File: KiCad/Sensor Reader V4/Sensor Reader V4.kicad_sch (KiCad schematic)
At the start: 33 parts, among them J1 ADS1115_HE_Reader, J10 Conn_01x02_Socket, J11 Conn_01x02_Socket, J12 Conn_01x02_Socket, J13 Conn_01x02_Socket, J14 Conn_01x02_Socket, J15 5V_Input, J16 3.3V_Output, J2 ADS1115_Battery_Voltage, J3 I2C Shifter High, J4 I2C Shifter Low, J5 USB_C_Receptacle_USB2.0_16P, J6 Exposed_UART, J7 Conn_01x02_Socket, J8 Conn_01x02_Socket, J9 Conn_01x02_Socket, SW1 SW_MEC_5E, SW2 SW_MEC_5E, U1 AMS1117-3.3, U2 USBLC6-2P6, U4 ESP32-C3-WROOM-02

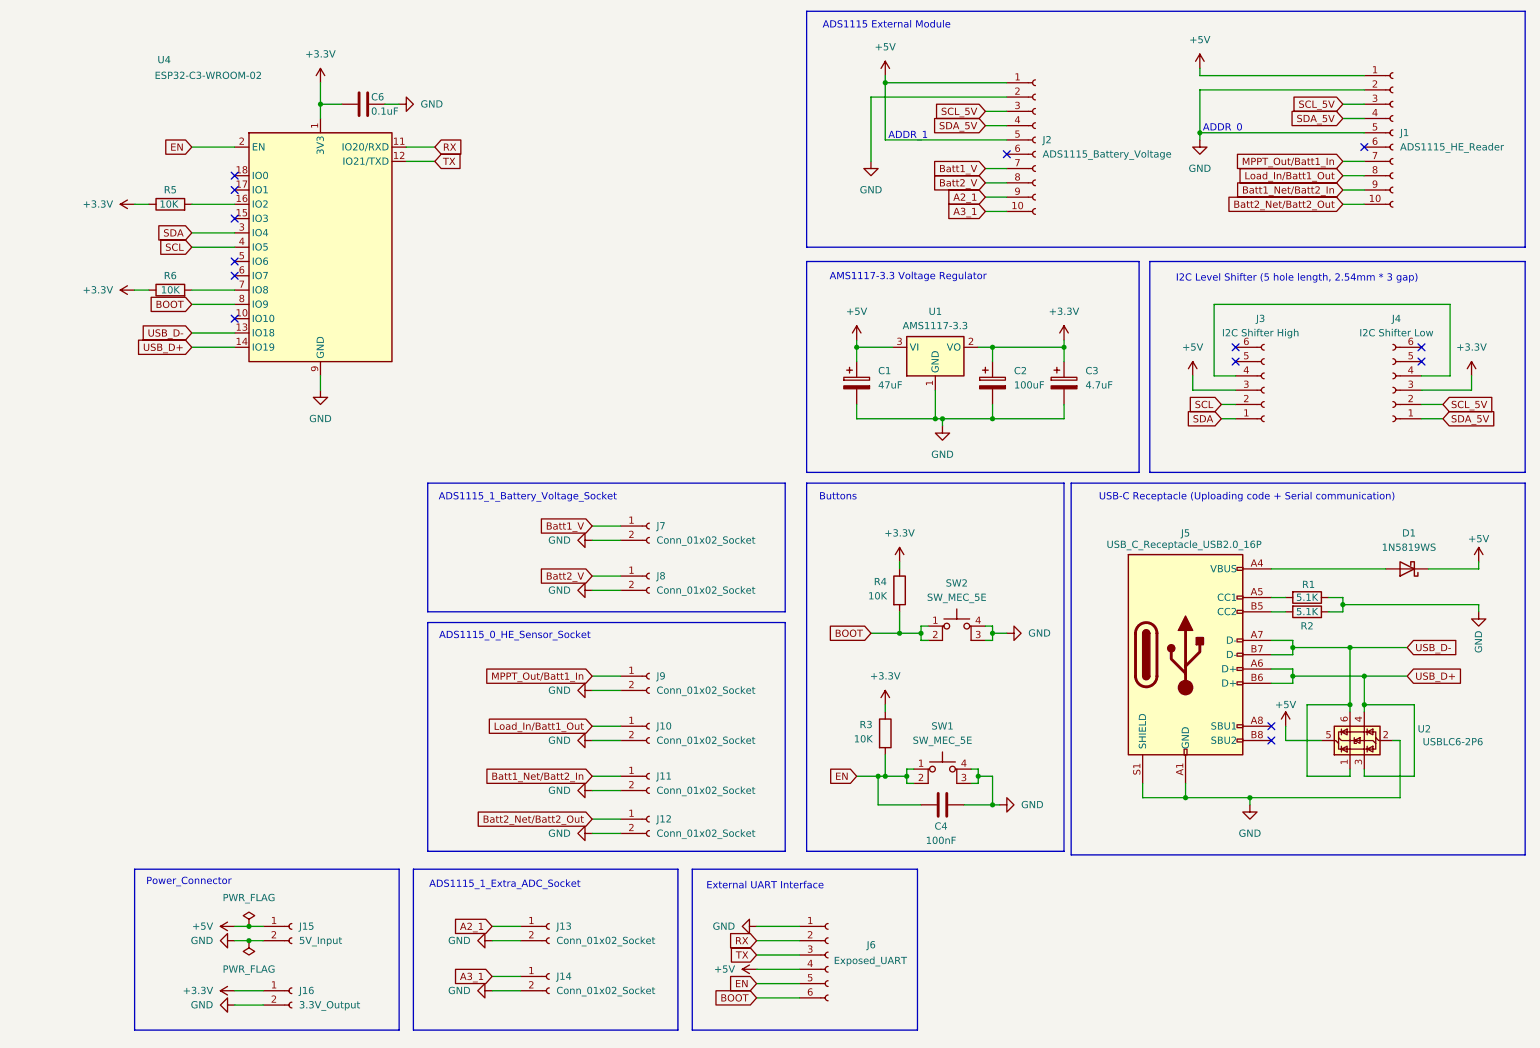
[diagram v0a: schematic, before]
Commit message: i
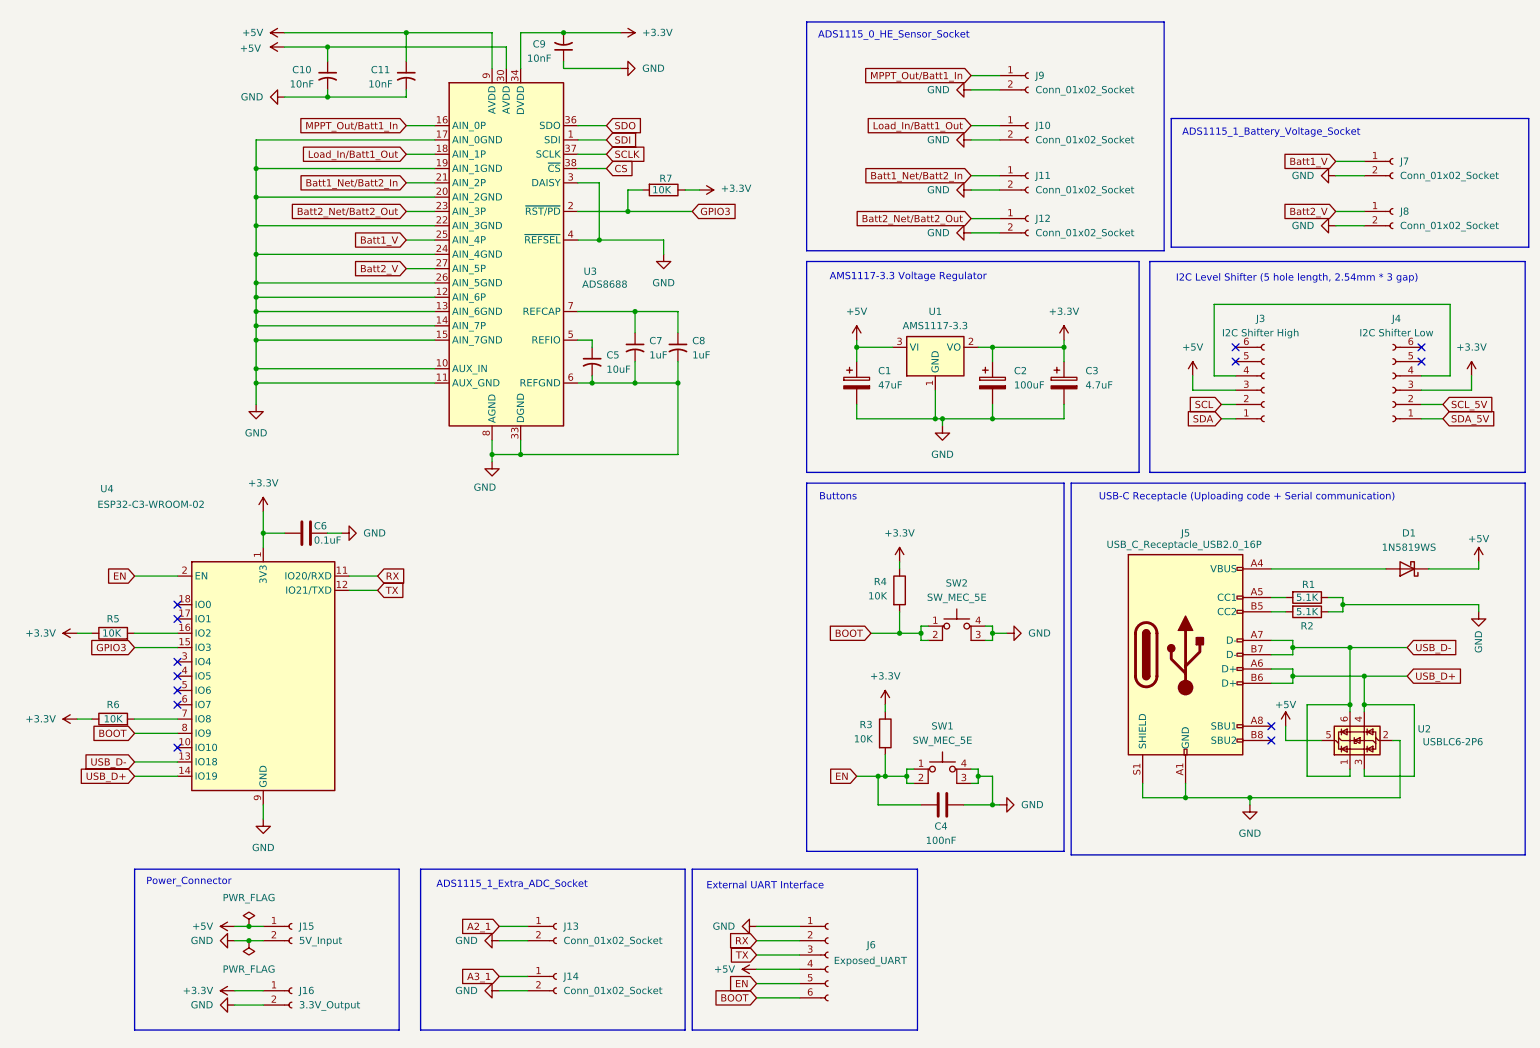
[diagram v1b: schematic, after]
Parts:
- removed J1: ADS1115_HE_Reader, symbol Connector:Conn_01x10_Socket
- removed J2: ADS1115_Battery_Voltage, symbol Connector:Conn_01x10_Socket
- added C10, C11, C9: 10nF, symbol Device:C_Small_US
- added C5: 10uF, symbol Device:C_Small_US
- added C7, C8: 1uF, symbol Device:C_Small_US
- added R7: 10K, symbol Device:R
- added U3: ADS8688, Package_SO:TSSOP-38_4.4x9.7mm_P0.5mm, symbol Analog_ADC:ADS8688
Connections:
- net +3.3V: now also C9.2, R7.1, U3.34 (DVDD)
- net +5V: now also C10.1, C11.1, U3.30 (AVDD), U3.9 (AVDD)
- net Batt1_Net/Batt2_In: now also U3.21 (AIN_2P)
- net Batt1_V: now also U3.25 (AIN_4P)
- net Batt2_Net/Batt2_Out: now also U3.23 (AIN_3P)
- net Batt2_V: now also U3.27 (AIN_5P)
- net GND: now also C10.2, C11.2, C5.2, C7.2, C8.2, C9.1, U3.10 (AUX_IN), U3.11 (AUX_GND), U3.12 (AIN_6P), U3.13 (AIN_6GND), U3.14 (AIN_7P), U3.15 (AIN_7GND), U3.17 (AIN_0GND), U3.19 (AIN_1GND), U3.20 (AIN_2GND), U3.22 (AIN_3GND), U3.24 (AIN_4GND), U3.26 (AIN_5GND), U3.28 (AGND), U3.29 (AGND), U3.3 (DAISY), U3.31 (AGND), U3.32 (AGND), U3.33 (DGND), U3.4 (~{REFSEL}), U3.6 (REFGND), U3.8 (AGND)
- net Load_In/Batt1_Out: now also U3.18 (AIN_1P)
- net MPPT_Out/Batt1_In: now also U3.16 (AIN_0P)
- net SCL: no longer U4.4 (IO5)
- net SDA: no longer U4.3 (IO4)
- net GPIO3: now reaches U4.15 (IO3)
- net GPIO3: now also R7.2, U3.2 (~{RST/PD})
- new net: C5.1, U3.5 (REFIO)
- new net: C7.1, C8.1, U3.7 (REFCAP)
- new net CS: U3.38 (~{CS})
- new net SCLK: U3.37 (SCLK)
- new net SDI: U3.1 (SDI)
- new net SDO: U3.36 (SDO)
- no-connect marks 14 -> 13
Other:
- note removed: "ADDR_0"
- note removed: "ADDR_1"
- note removed: "ADS1115 External Module"
- moved on the sheet: C6, J10, J11, J12, J13, J14, J7, J8, J9, R5, R6, U4

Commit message: finish populating components
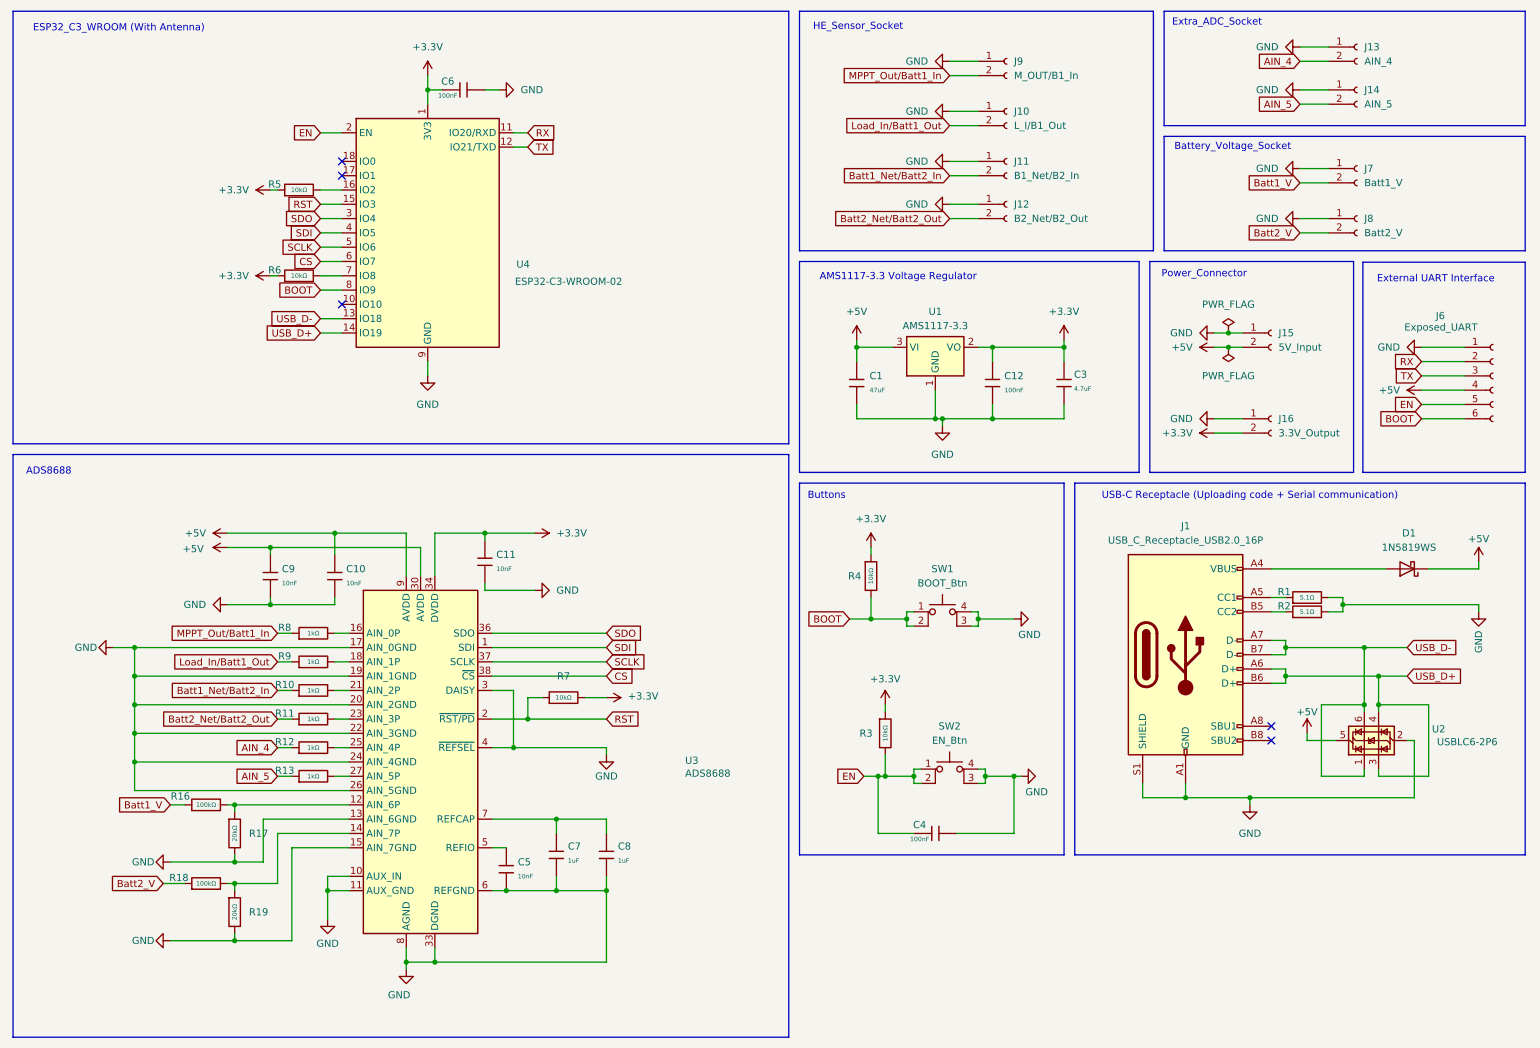
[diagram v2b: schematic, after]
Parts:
- removed C1: 47uF, symbol Device:C_Polarized
- removed C10, C11, C9: 10nF, symbol Device:C_Small_US
- removed C2: 100uF, symbol Device:C_Polarized
- removed C3: 4.7uF, symbol Device:C_Polarized
- removed C4: 100nF, symbol Device:C
- removed C5: 10uF, symbol Device:C_Small_US
- removed C6: 0.1uF, symbol Device:C
- removed C7, C8: 1uF, symbol Device:C_Small_US
- removed J3: I2C Shifter High, symbol Connector:Conn_01x06_Socket
- removed J4: I2C Shifter Low, symbol Connector:Conn_01x06_Socket
- removed J5: USB_C_Receptacle_USB2.0_16P, symbol Connector:USB_C_Receptacle_USB2.0_16P
- removed R1, R2: 5.1K, symbol Device:R
- removed R3, R4, R5, R6, R7: 10K, symbol Device:R
- added C1: 47uF, PCM_JLCPCB:C_0805, symbol PCM_JLCPCB-Capacitors:0805,47uF
- added C10, C11, C5, C9: 10nF, PCM_JLCPCB:C_0603, symbol PCM_JLCPCB-Capacitors:0603,10nF
- added C12, C4, C6: 100nF, PCM_JLCPCB:C_0603, symbol PCM_JLCPCB-Capacitors:0603,100nF
- added C3: 4.7uF, PCM_JLCPCB:C_0603, symbol PCM_JLCPCB-Capacitors:0603,4.7uF
- added C7, C8: 1uF, PCM_JLCPCB:C_0603, symbol PCM_JLCPCB-Capacitors:0603,1uF
- added J1: USB_C_Receptacle_USB2.0_16P, Connector_USB:USB_C_Receptacle_Palconn_UTC16-G, symbol Connector:USB_C_Receptacle_USB2.0_16P
- added R1, R2: 5.1Ω, PCM_JLCPCB:R_0603, symbol PCM_JLCPCB-Resistors:0603,5.1Ω
- added R10, R11, R12, R13, R8, R9: 1kΩ, PCM_JLCPCB:R_0603, symbol PCM_JLCPCB-Resistors:0603,1kΩ
- added R16, R18: 100kΩ, PCM_JLCPCB:R_0603, symbol PCM_JLCPCB-Resistors:0603,100kΩ
- added R17, R19: 20kΩ, PCM_JLCPCB:R_0603, symbol PCM_JLCPCB-Resistors:0603,20kΩ
- added R3, R4, R5, R6, R7: 10kΩ, PCM_JLCPCB:R_0603, symbol PCM_JLCPCB-Resistors:0603,10kΩ
- J10: value Conn_01x02_Socket -> L_I/B1_Out; footprint (none) -> Connector_JST:JST_XH_B2B-XH-A_1x02_P2.50mm_Vertical
- J11: value Conn_01x02_Socket -> B1_Net/B2_In; footprint (none) -> Connector_JST:JST_XH_B2B-XH-A_1x02_P2.50mm_Vertical
- J12: value Conn_01x02_Socket -> B2_Net/B2_Out; footprint (none) -> Connector_JST:JST_XH_B2B-XH-A_1x02_P2.50mm_Vertical
- J13: value Conn_01x02_Socket -> AIN_4; footprint (none) -> Connector_JST:JST_XH_B2B-XH-A_1x02_P2.50mm_Vertical
- J14: value Conn_01x02_Socket -> AIN_5; footprint (none) -> Connector_JST:JST_XH_B2B-XH-A_1x02_P2.50mm_Vertical
- J15: footprint (none) -> Connector_JST:JST_XH_B2B-XH-A_1x02_P2.50mm_Vertical
- J16: footprint (none) -> Connector_PinHeader_2.54mm:PinHeader_1x02_P2.54mm_Vertical
- J6: footprint (none) -> Connector_PinHeader_2.54mm:PinHeader_1x06_P2.54mm_Vertical
- J7: value Conn_01x02_Socket -> Batt1_V; footprint (none) -> Connector_JST:JST_XH_B2B-XH-A_1x02_P2.50mm_Vertical
- J8: value Conn_01x02_Socket -> Batt2_V; footprint (none) -> Connector_JST:JST_XH_B2B-XH-A_1x02_P2.50mm_Vertical
- J9: value Conn_01x02_Socket -> M_OUT/B1_In; footprint (none) -> Connector_JST:JST_XH_B2B-XH-A_1x02_P2.50mm_Vertical
- SW1: value SW_MEC_5E -> BOOT_Btn; footprint Button_Switch_SMD:SW_MEC_5GSH9 -> PCM_JLCPCB:SW-SMD_4P-L5.1-W5.1-P3.70-LS6.5-TL-2
- SW2: value SW_MEC_5E -> EN_Btn; footprint Button_Switch_SMD:SW_MEC_5GSH9 -> PCM_JLCPCB:SW-SMD_4P-L5.1-W5.1-P3.70-LS6.5-TL-2
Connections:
- net A2_1 is gone; now on net GND: J13.1 (Pin_1)
- net A3_1 is gone; now on net GND: J14.1 (Pin_1)
- net +3.3V: now also J16.2 (Pin_2), C11.1, C12.2, C3.1, C6.1, R3.1, R4.1, R5.1, R6.1, R7.2; no longer J16.1 (Pin_1)
- net +5V: now also J15.2 (Pin_2), C1.1, C10.1, C9.1; no longer J15.1 (Pin_1)
- net BOOT: now also SW1.1, SW1.2, R4.2; no longer SW2.1, SW2.2
- net Batt1_Net/Batt2_In: now also J11.2 (Pin_2), R10.1; no longer J11.1 (Pin_1), U3.21 (AIN_2P)
- net Batt1_V: now also J7.2 (Pin_2), R16.1; no longer J7.1 (Pin_1), U3.25 (AIN_4P)
- net Batt2_Net/Batt2_Out: now also J12.2 (Pin_2), R11.1; no longer J12.1 (Pin_1), U3.23 (AIN_3P)
- net Batt2_V: now also J8.2 (Pin_2), R18.1; no longer J8.1 (Pin_1), U3.27 (AIN_5P)
- net CS: now also U4.6 (IO7)
- net EN: now also SW2.1, SW2.2, C4.1, R3.2; no longer SW1.1, SW1.2
- net GND: now also J10.1 (Pin_1), J11.1 (Pin_1), J12.1 (Pin_1), J15.1 (Pin_1), J16.1 (Pin_1), J7.1 (Pin_1), J8.1 (Pin_1), J9.1 (Pin_1), C1.2, C10.2, C11.2, C12.1, C3.2, C4.2, C5.2, C6.2, C7.2, C8.2, C9.2, J1.A1 (GND), J1.A12 (GND), J1.B1 (GND), J1.B12 (GND), J1.S1 (SHIELD), R1.2, R17.2, R19.2, R2.2; no longer J10.2 (Pin_2), J11.2 (Pin_2), J12.2 (Pin_2), J13.2 (Pin_2), J14.2 (Pin_2), J15.2 (Pin_2), J16.2 (Pin_2), J7.2 (Pin_2), J8.2 (Pin_2), J9.2 (Pin_2), U3.12 (AIN_6P), U3.14 (AIN_7P)
- net Load_In/Batt1_Out: now also J10.2 (Pin_2), R9.1; no longer J10.1 (Pin_1), U3.18 (AIN_1P)
- net MPPT_Out/Batt1_In: now also J9.2 (Pin_2), R8.1; no longer J9.1 (Pin_1), U3.16 (AIN_0P)
- net SCLK: now also U4.5 (IO6)
- net SDI: now also U4.4 (IO5)
- net SDO: now also U4.3 (IO4)
- net USB_D+: now also J1.A6 (D+), J1.B6 (D+)
- net USB_D-: now also J1.A7 (D-), J1.B7 (D-)
- net at U3.5 (REFIO): now also C5.1
- net at U3.7 (REFCAP): now also C7.1, C8.1
- net at D1.2 (A): now also J1.A4 (VBUS), J1.A9 (VBUS), J1.B4 (VBUS), J1.B9 (VBUS)
- net at U4.7 (IO8): now also R6.2
- net at U4.16 (IO2): now also R5.2
- net GPIO3 renamed RST
- net RST: now also R7.1
- new net: R11.2, U3.23 (AIN_3P)
- new net: R18.2, R19.1, U3.14 (AIN_7P)
- new net: R10.2, U3.21 (AIN_2P)
- new net: R16.2, R17.1, U3.12 (AIN_6P)
- new net: R8.2, U3.16 (AIN_0P)
- new net: R9.2, U3.18 (AIN_1P)
- new net: R12.2, U3.25 (AIN_4P)
- new net: R13.2, U3.27 (AIN_5P)
- new net: J1.A5 (CC1), R1.1
- new net: J1.B5 (CC2), R2.1
- new net AIN_4: J13.2 (Pin_2), R12.1
- new net AIN_5: J14.2 (Pin_2), R13.1
- no-connect marks 13 -> 5
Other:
- note added: "ADS8688"
- note added: "Battery_Voltage_Socket"
- note added: "ESP32_C3_WROOM (With Antenna)"
- note added: "Extra_ADC_Socket"
- note added: "HE_Sensor_Socket"
- note removed: "ADS1115_0_HE_Sensor_Socket"
- note removed: "ADS1115_1_Battery_Voltage_Socket"
- note removed: "ADS1115_1_Extra_ADC_Socket"
- note removed: "I2C Level Shifter (5 hole length, 2.54mm * 3 gap)"
- moved on the sheet: J10, J11, J12, J13, J14, J15, J16, J6, J7, J8, J9, U2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
